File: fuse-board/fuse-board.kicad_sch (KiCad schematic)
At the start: 21 parts, among them J2 74651173R, J3 74651173R, J4 ATM15-12PA-BM04, J5 1053141106, U2 AP63205WU, U3 MIC5504-3.3YM5

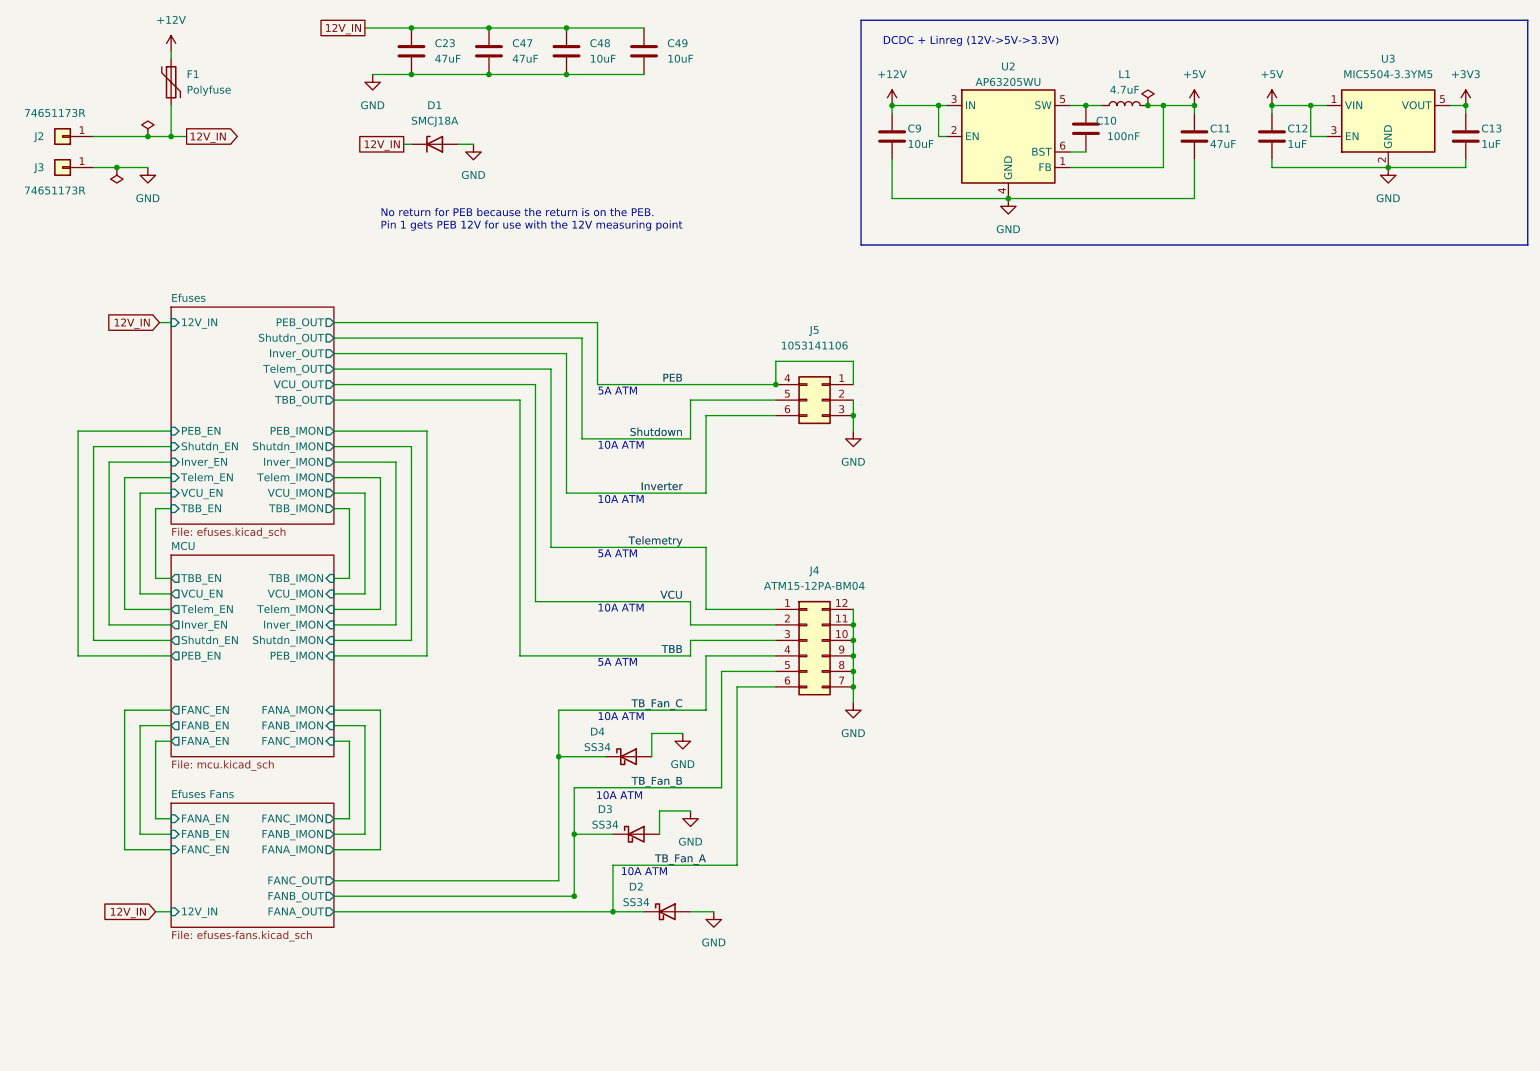
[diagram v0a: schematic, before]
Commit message: add sheet pins and status LEDs
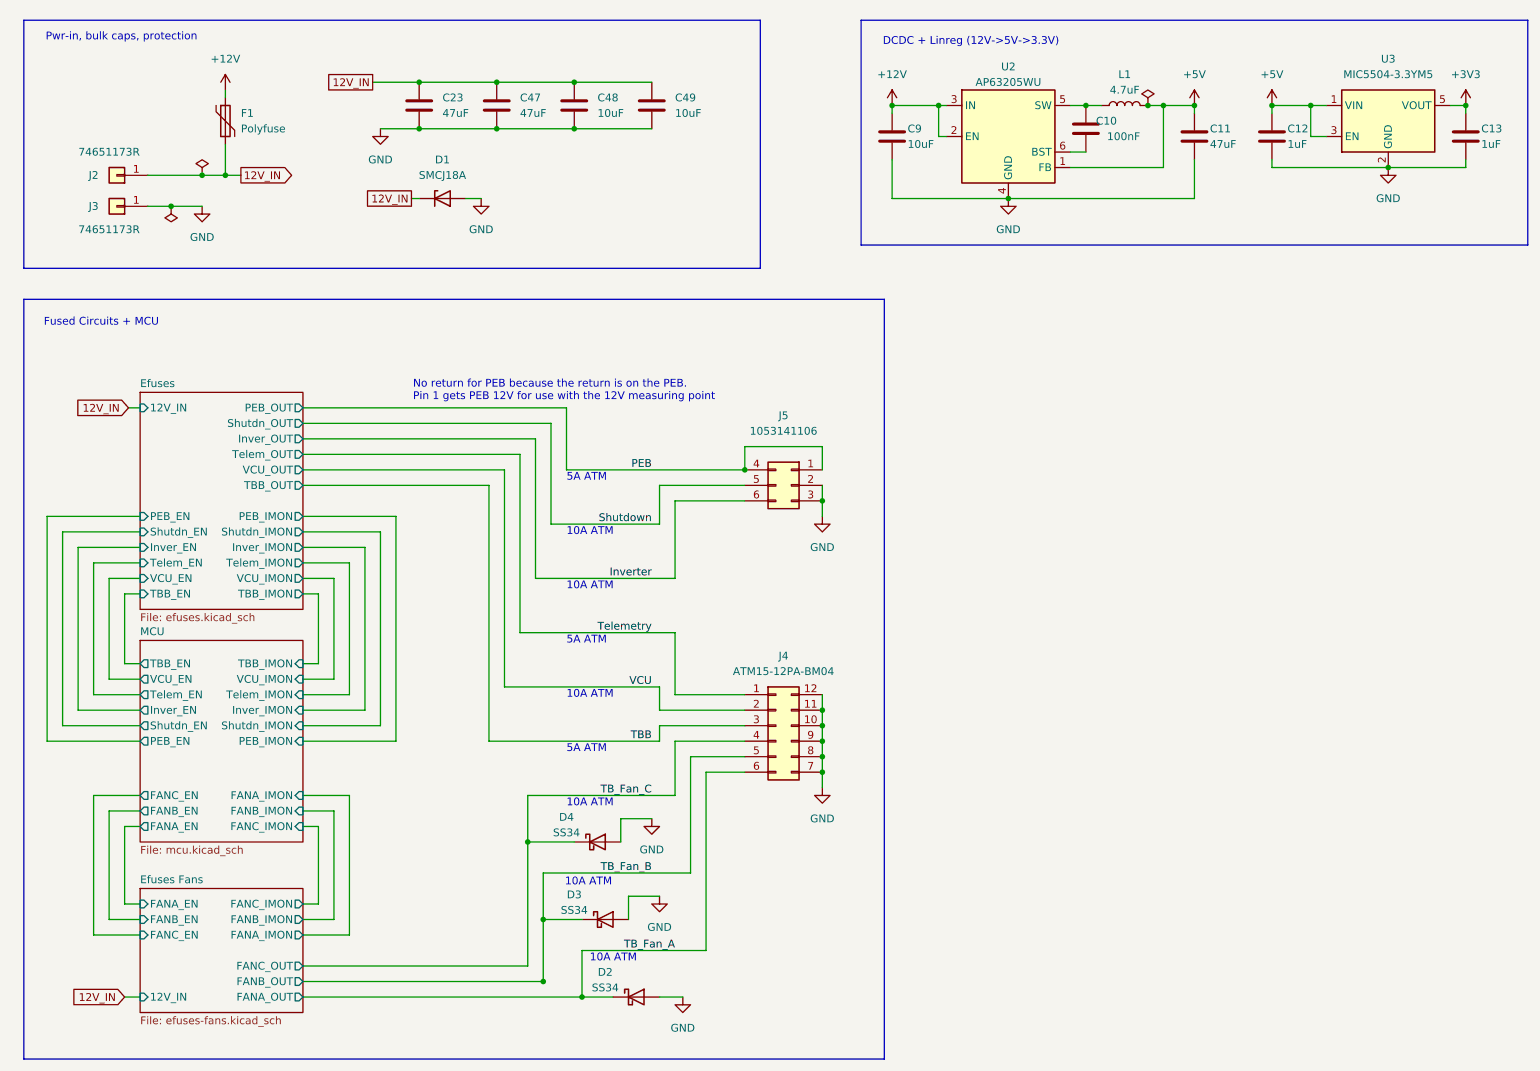
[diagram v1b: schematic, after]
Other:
- note added: "Fused Circuits + MCU"
- note added: "Pwr-in, bulk caps, protection"
- moved on the sheet: C23, C47, C48, C49, D1, D2, D3, D4, F1, J2, J3, J4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

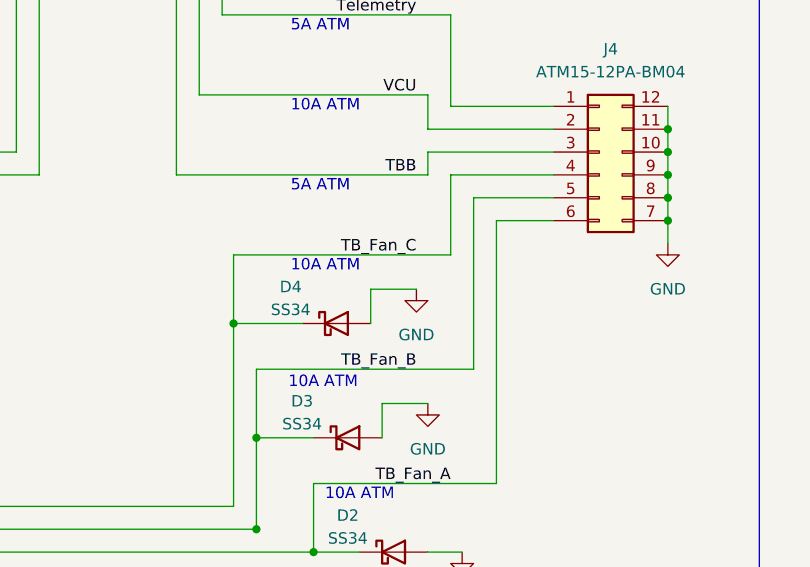
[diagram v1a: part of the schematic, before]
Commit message: fix weird unconnected wire
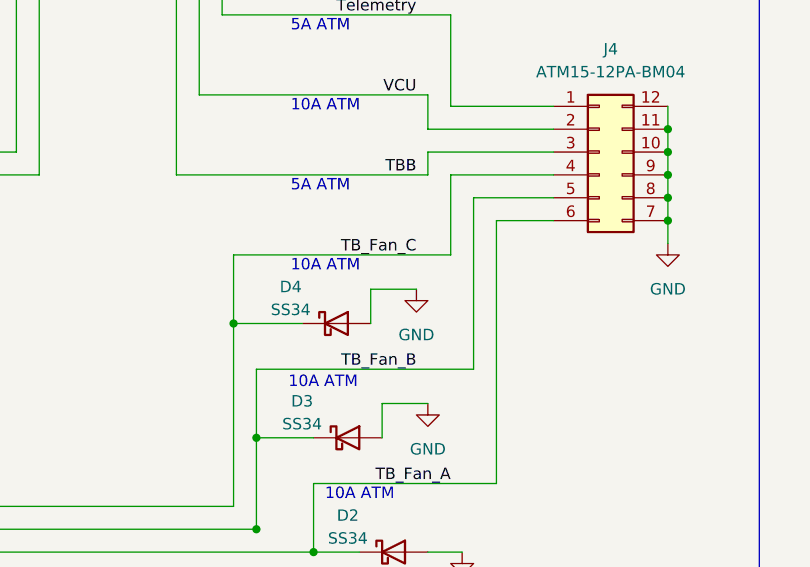
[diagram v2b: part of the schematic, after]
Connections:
- net Efuses Fans/FANB_OUT is gone; now on net TB_Fan_B: D3.1 (K)
